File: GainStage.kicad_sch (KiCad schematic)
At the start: 30 parts, among them U1 LTC6269 A, U2 LTC6269 A, U3 LTC6268IS6

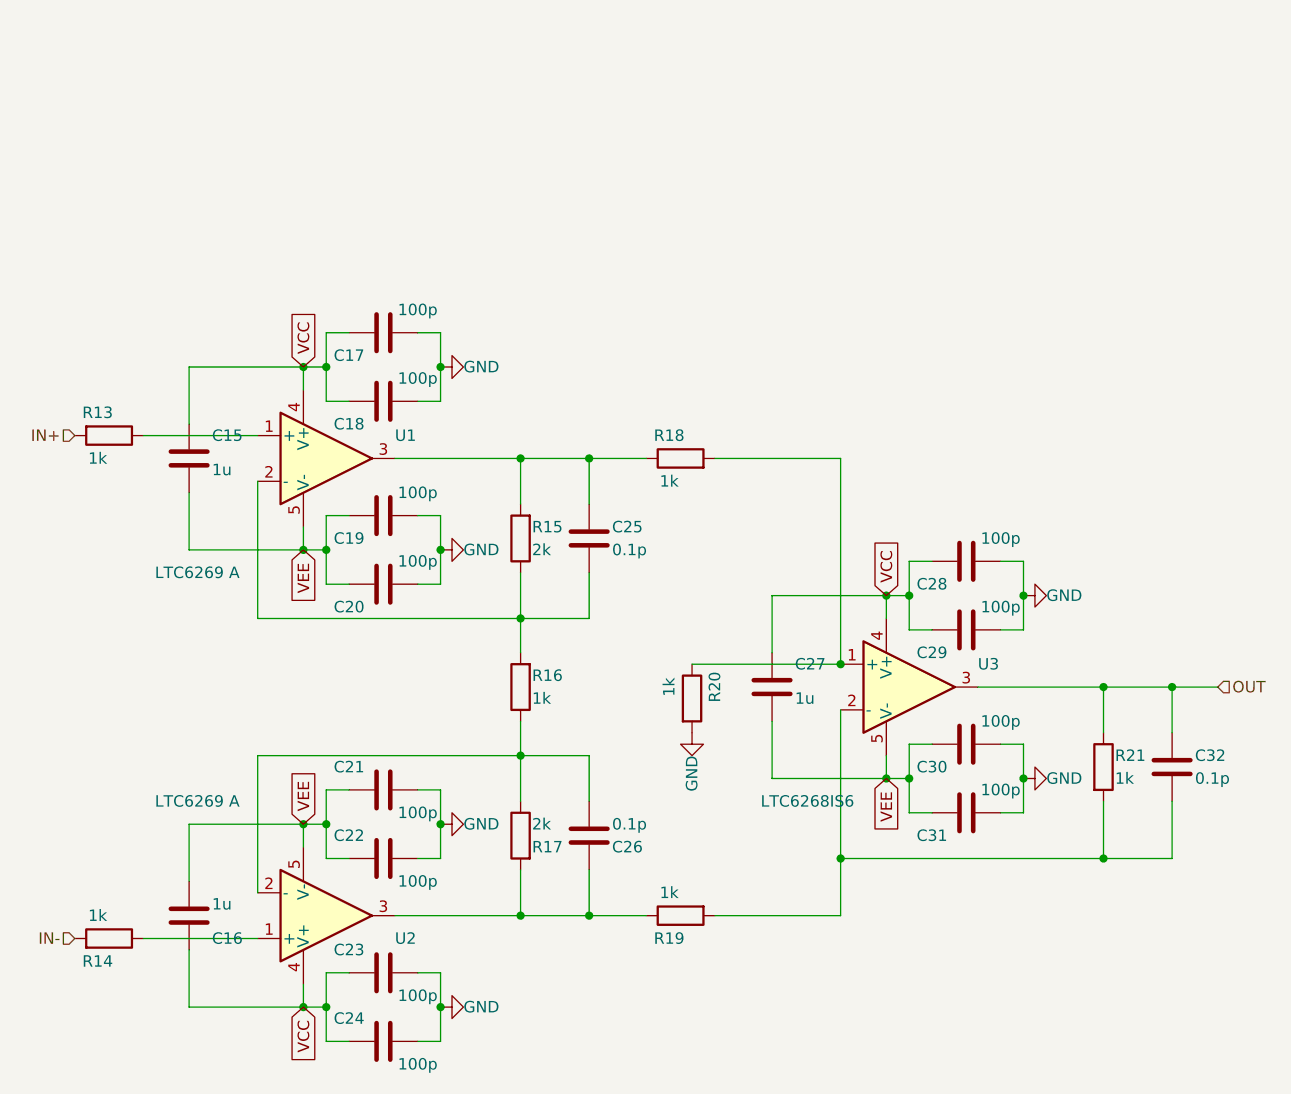
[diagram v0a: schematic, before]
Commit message: Routed PCB
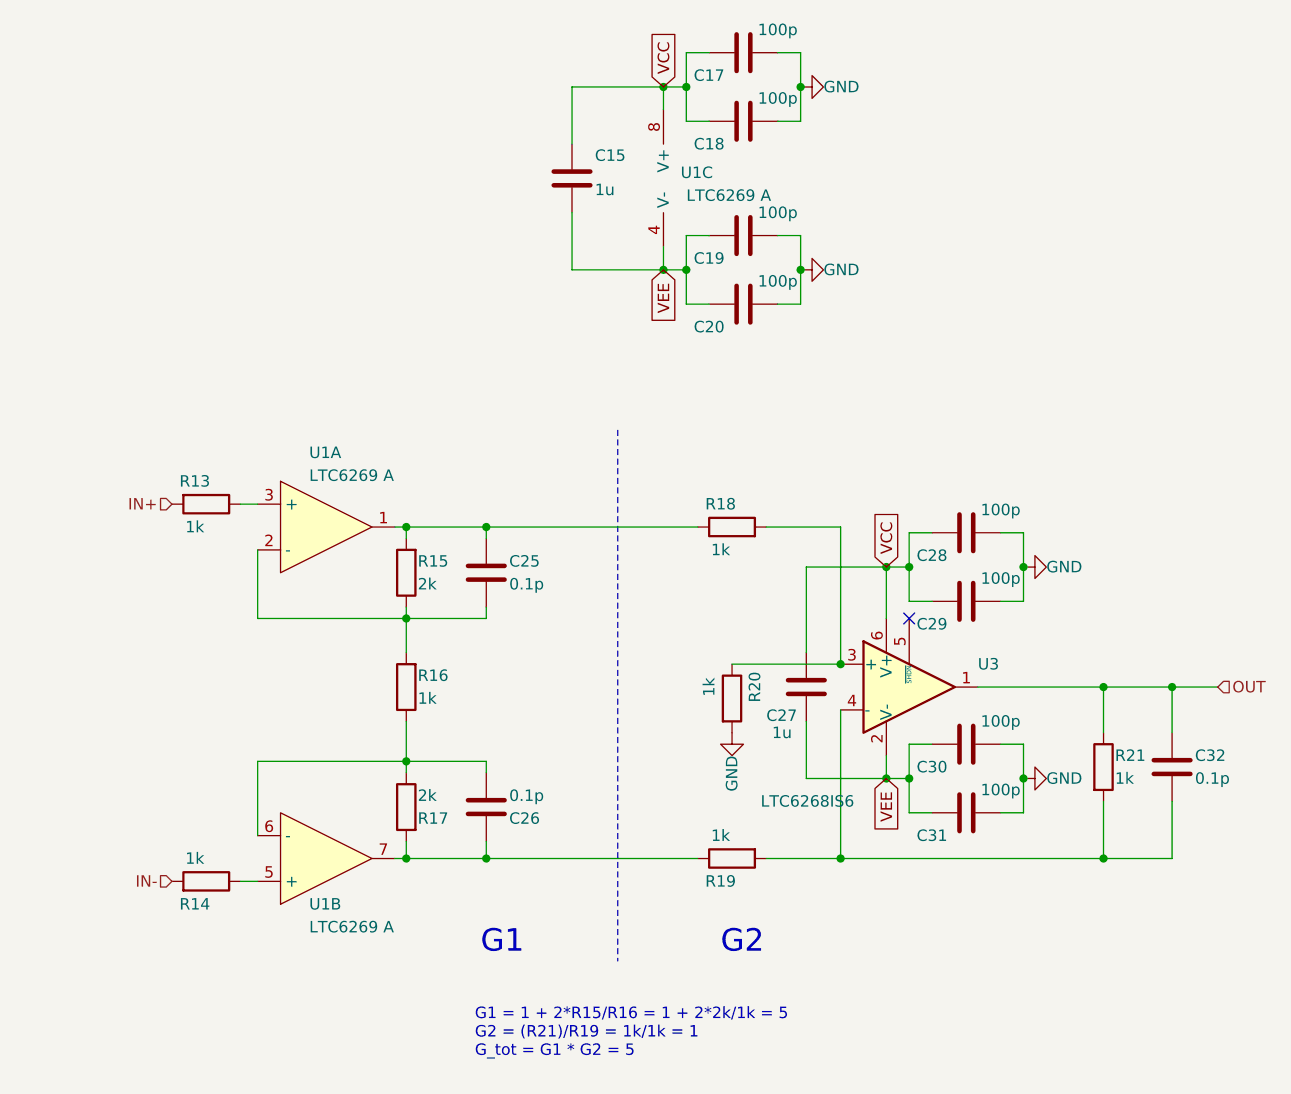
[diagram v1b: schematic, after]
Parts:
- removed C16: 1u, Capacitor_SMD:C_0603_1608Metric, symbol Device:C
- removed C21, C22, C23, C24: 100p, Capacitor_SMD:C_0603_1608Metric, symbol Device:C
- added unit 3 of U1
- U1: footprint Package_SO:SOIC-8-1EP_3.9x4.9mm_P1.27mm_EP2.29x3mm -> Package_SO:MSOP-8-1EP_3x3mm_P0.65mm_EP1.68x1.88mm; symbol pspice:OPAMP -> Amplifier_Operational:LTC6269xMS8E
- U1: renamed from U2; footprint Package_SO:SOIC-8-1EP_3.9x4.9mm_P1.27mm_EP2.29x3mm -> Package_SO:MSOP-8-1EP_3x3mm_P0.65mm_EP1.68x1.88mm; symbol pspice:OPAMP -> Amplifier_Operational:LTC6269xMS8E
- U3: footprint Package_SO:TSOP-6_1.65x3.05mm_P0.95mm -> Package_TO_SOT_SMD:TSOT-23-6; symbol pspice:OPAMP -> Amplifier_Operational:LTC6268xS6-10
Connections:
- net OUT: now also U3.1; no longer U3.3
- net VCC: now also U3.6 (V+), U1.8 (V+); no longer U1.4 (V+), U1.4 (V+), U3.4 (V+)
- net VEE: now also U3.2 (V-), U1.4 (V-), U1.9 (V-); no longer U1.5 (V-), U1.5 (V-), U3.5 (V-)
- net at R13.1: now also U1.3 (+); no longer U1.1 (+)
- net at C25.1, R15.2, R18.1: now also U1.1; no longer U1.3
- net at R18.2, R20.1: now also U3.3 (+); no longer U3.1 (+)
- net at C26.2, R16.1, R17.1: now also U1.6 (-); no longer U1.2 (-)
- net at C32.1, R19.2, R21.2: now also U3.4 (-); no longer U3.2 (-)
- net at R14.1: now also U1.5 (+); no longer U1.1 (+)
- net at C26.1, R17.2, R19.1: now also U1.7; no longer U1.3
- no-connect marks 0 -> 1
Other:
- note added: "G1"
- note added: "G1 = 1 + 2*R15/R16 = 1 + 2*2k/1k = 5 G2 = (R21)/R19 = 1k/1k = 1 G_tot = G1 * G2 = 5"
- note added: "G2"
- moved on the sheet: C15, C17, C18, C19, C20, C25, C26, C27, C28, C29, R13, R14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
